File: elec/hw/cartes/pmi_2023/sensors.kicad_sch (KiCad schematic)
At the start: 43 parts, among them U10 AD8531ARTZ, U11 GP2S60B, U12 GP2S60B, U13 GP2S60B, U14 GP2S60B, U15 GP2S60B, U16 GP2S60B, U17 GP2S60B, U18 GP2S60B, U19 tof_sensor_master, U20 tof_sensor_master, U21 tof_sensor_master, U22 tof_sensor_master, U23 tof_sensor_master, U24 tof_sensor_master, U25 tof_sensor_master, U26 tof_sensor_master

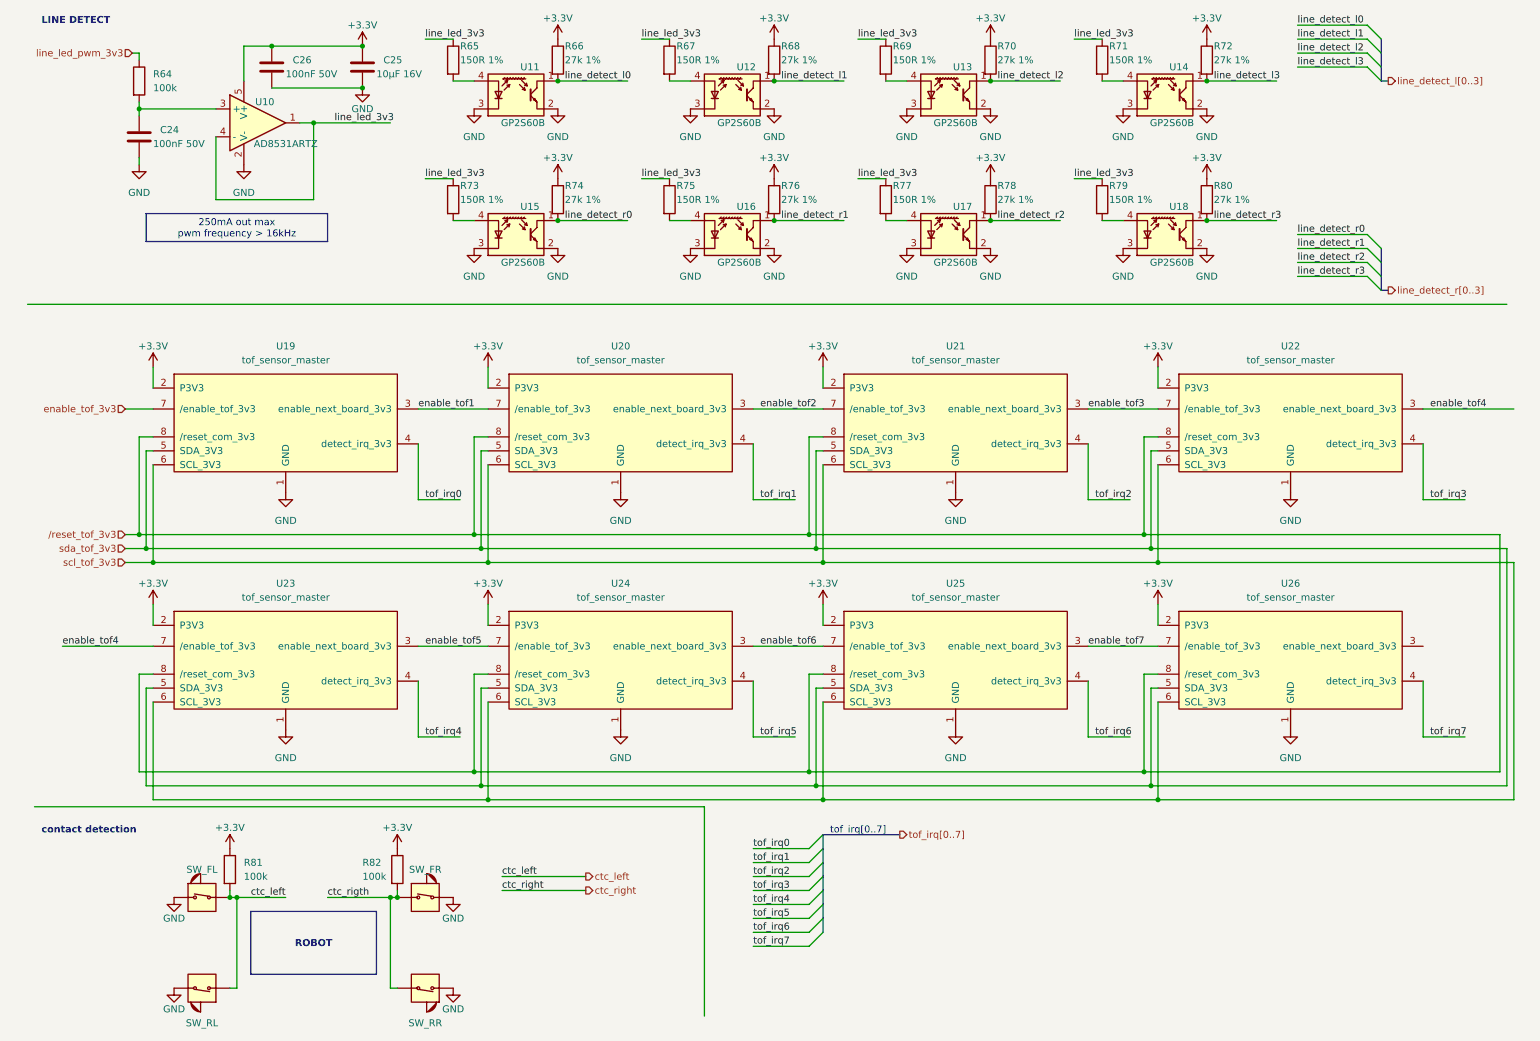
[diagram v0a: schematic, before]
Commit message: pmi2023 wip
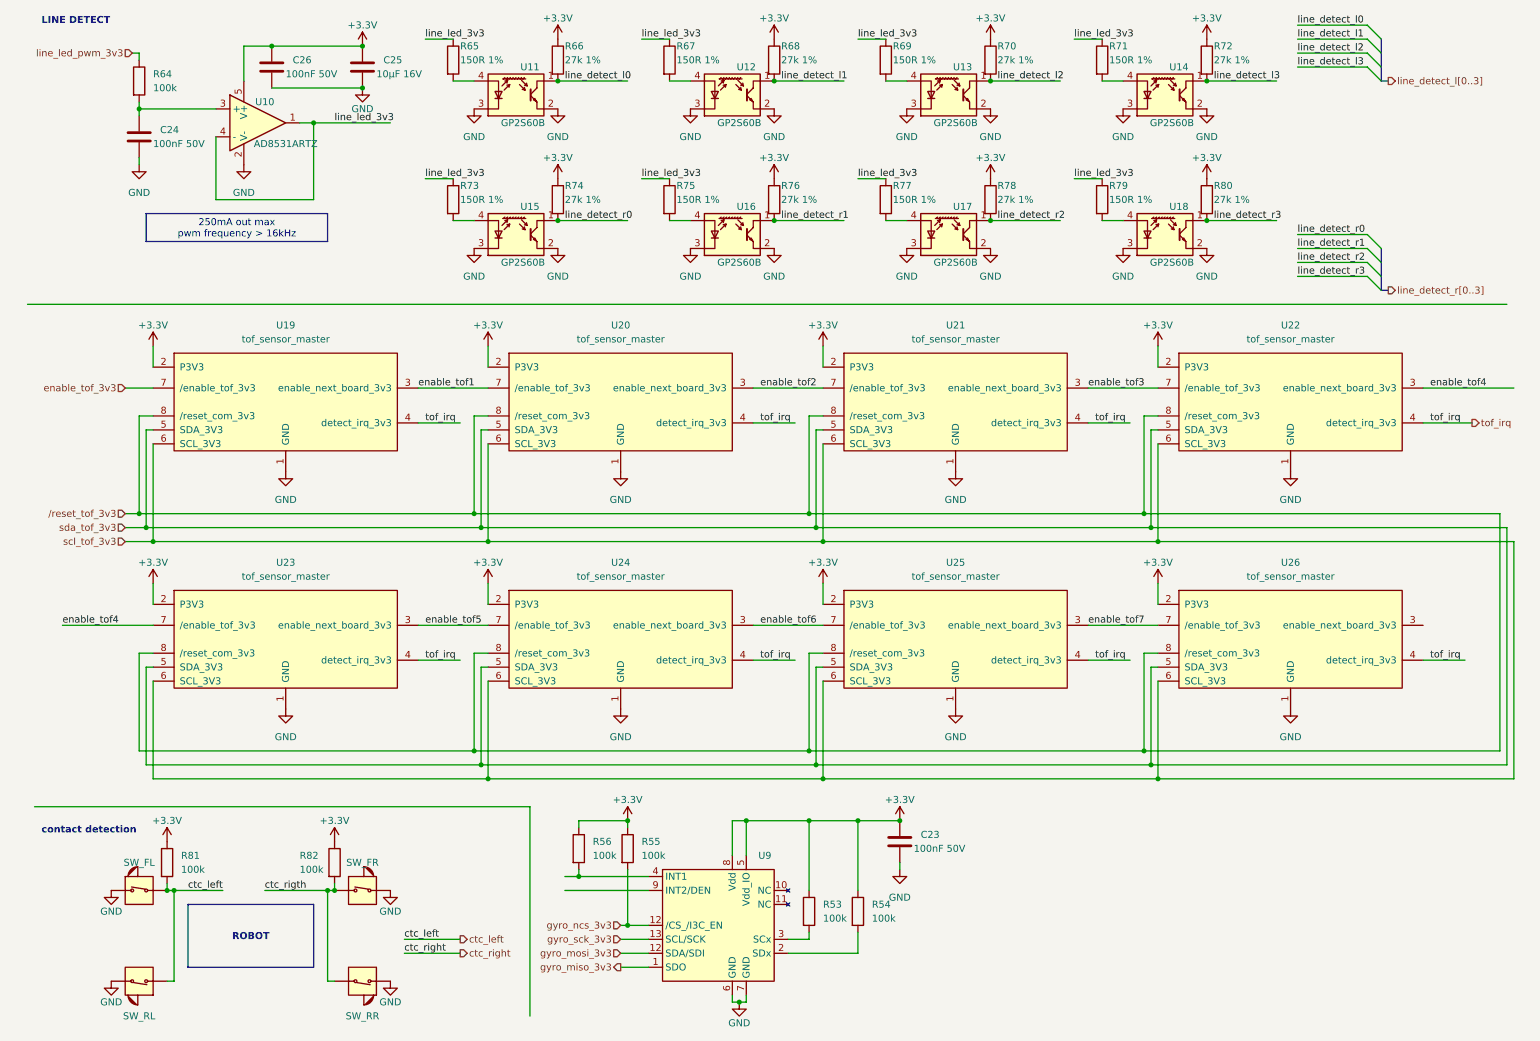
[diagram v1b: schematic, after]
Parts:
- added C23: 100nF 50V, symbol cocotter_capacitors:C_100nF_50V_0603
- added R53, R54, R55, R56: 100k, cocotter_resistor:r0603_reflow, symbol cocotter_resistors:R_100k_0603_1%
- added U9: ~, symbol cocotter_ic:LSM6DSO32XTR
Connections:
- net tof_irq1 is gone; now on net tof_irq: U20.4 (detect_irq_3v3)
- net tof_irq2 is gone; now on net tof_irq: U21.4 (detect_irq_3v3)
- net tof_irq3 is gone; now on net tof_irq: U22.4 (detect_irq_3v3)
- net tof_irq4 is gone; now on net tof_irq: U23.4 (detect_irq_3v3)
- net tof_irq5 is gone; now on net tof_irq: U24.4 (detect_irq_3v3)
- net tof_irq6 is gone; now on net tof_irq: U25.4 (detect_irq_3v3)
- net tof_irq7 is gone; now on net tof_irq: U26.4 (detect_irq_3v3)
- net +3.3V: now also C23.1, R53.1, R54.1, R55.1, R56.1, U9.5 (Vdd_IO), U9.8 (Vdd)
- net GND: now also C23.2, U9.6 (GND), U9.7 (GND)
- net tof_irq0 renamed tof_irq
- new net: R53.2, U9.3 (SCx)
- new net: R56.2, U9.4 (INT1)
- new net: R54.2, U9.2 (SDx)
- new net gyro_miso_3v3: U9.1 (SDO)
- new net gyro_mosi_3v3: U9.12 (SDA/SDI)
- new net gyro_ncs_3v3: R55.2, U9.12 (SDA/SDI)
- new net gyro_sck_3v3: U9.13 (SCL/SCK)
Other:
- note removed: "tof_irq[0..7]"
- moved on the sheet: R81, R82, SW_FL, SW_FR, SW_RL, SW_RR, U19, U20, U21, U22, U23, U24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
